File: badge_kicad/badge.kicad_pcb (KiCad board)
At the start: 2 copper layers, 76.9 x 42.2 mm, 19 parts, among them P2 Pin, P3 Pin, P4 Pin, P5 Pin, P6 Pin, SW1 ON

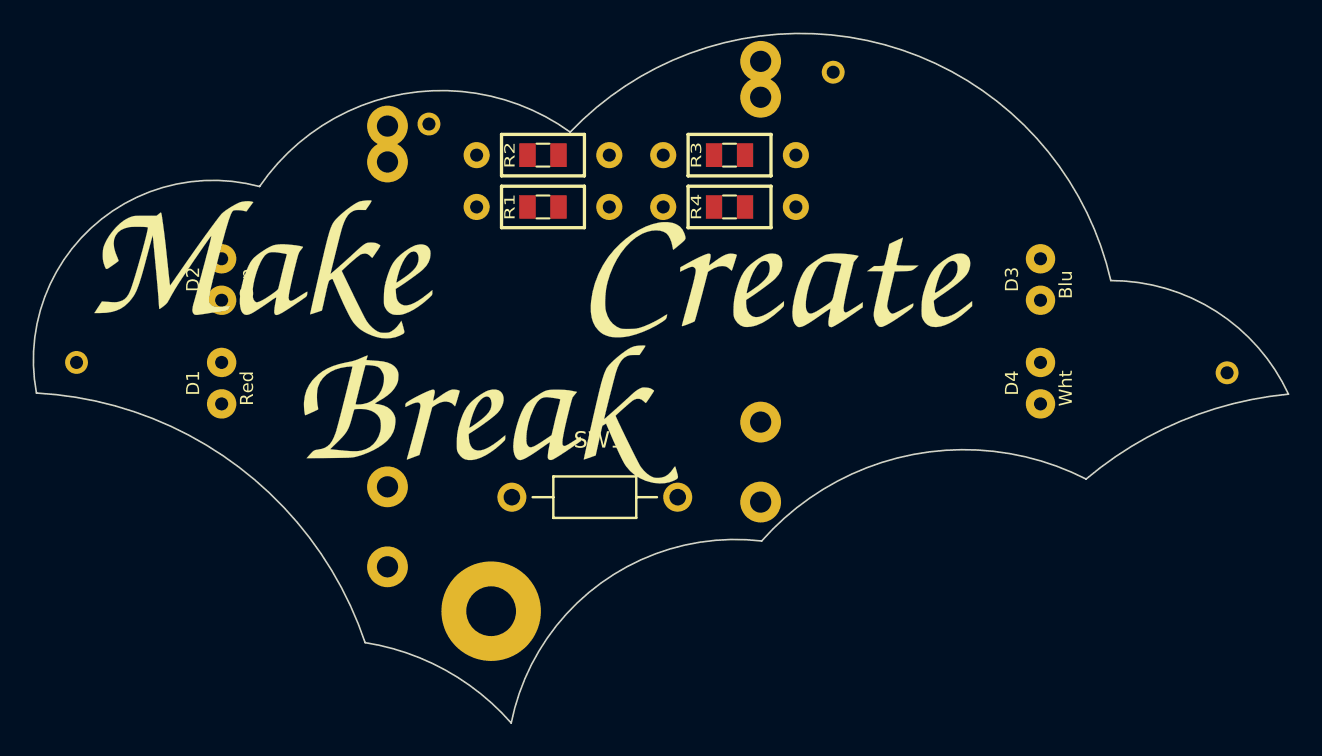
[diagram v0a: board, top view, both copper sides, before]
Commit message: rev2 mockup
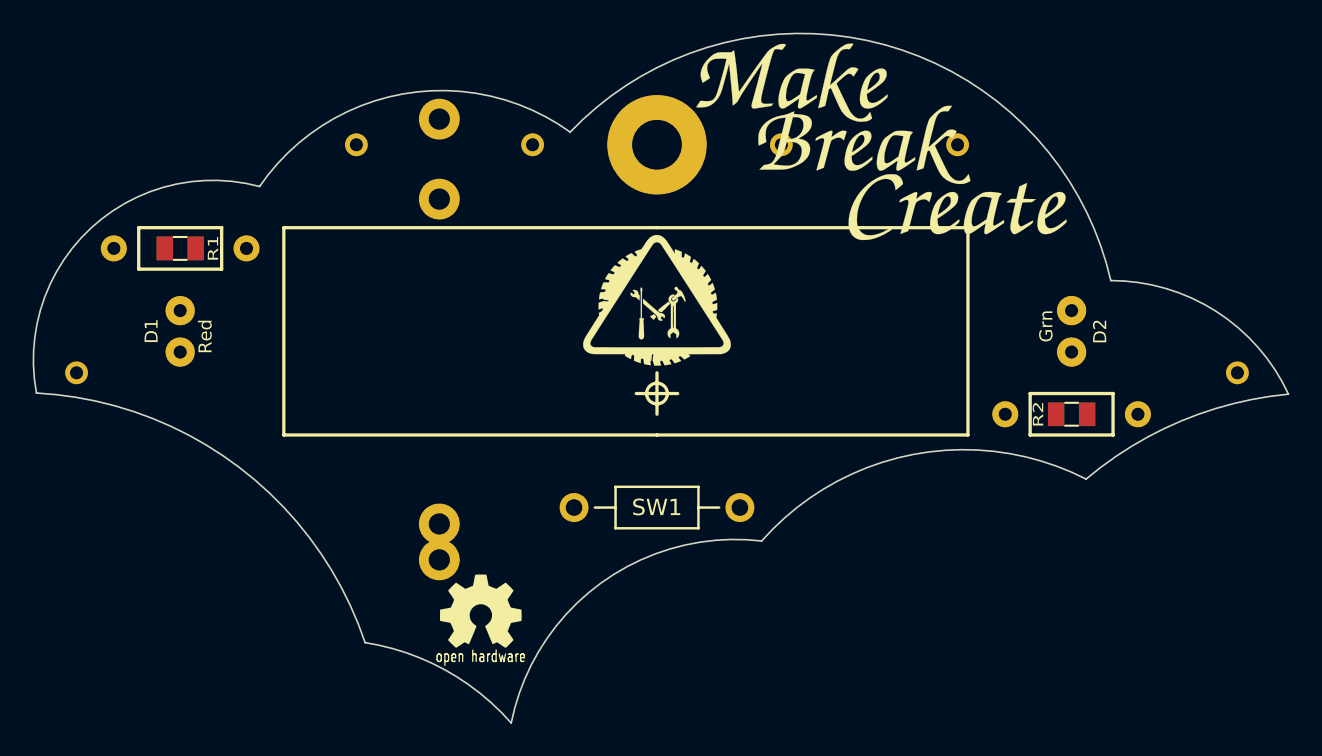
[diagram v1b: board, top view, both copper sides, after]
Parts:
- removed BT2: BATT_2, badge_fp:cr2032_02
- removed D3: Blu, badge_fp:LED-5MM
- removed D4: Wht, badge_fp:LED-5MM
- removed the G*** at (36.8, 43.2)
- removed the G*** at (50.8, 52.1)
- removed the G*** at (68.6, 43.8)
- removed R3, R4: 10E, badge_fp:r_0805
- added G***: LOGO, badge_fp:create3, F.Cu at (79.4, 39.4)
- added G***: LOGO, badge_fp:make3, F.Cu at (69.2, 31.8)
- added G***: LOGO, badge_fp:break3, F.Cu at (73.7, 35.6)
- added G***: LOGO, badge_fp:Logo_silk_OSHW_6x6mm, F.Cu at (50.2, 64.1)
- added G***: LOGO, badge_fp:MA_LOGO10, F.Cu at (61.0, 45.1)
- added P4: Pin, badge_fp:MTG_0mm8, F.Cu at (96.5, 49.5)
- added P5: Pin, badge_fp:MTG_0mm8, F.Cu at (42.5, 35.6)
- moved D2 52.2 mm to (86.4, 47.0), turned to 90 degrees
- moved R2 36.1 mm to (86.4, 52.1)
- moved P2 30.3 mm to (61.0, 35.6)
- moved R1 22.4 mm to (31.8, 41.9), turned to 180 degrees
- moved P6 21.6 mm to (79.4, 35.6)
- moved P5 6.48 mm to (53.3, 35.6)
- moved P3 5.46 mm to (68.6, 35.6)
- moved D1 4.07 mm to (31.8, 47.0)
- moved SW1 3.86 mm to (61.0, 57.8)
- moved BT1 3.48 mm to (47.6, 47.0), turned to 180 degrees
- moved P4 0.63 mm to (25.4, 49.5)
